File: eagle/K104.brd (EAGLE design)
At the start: 428.3 x 123.6 mm, 229 parts, among them IC1 MAX7219CNG, IC2 MAX7219CNG

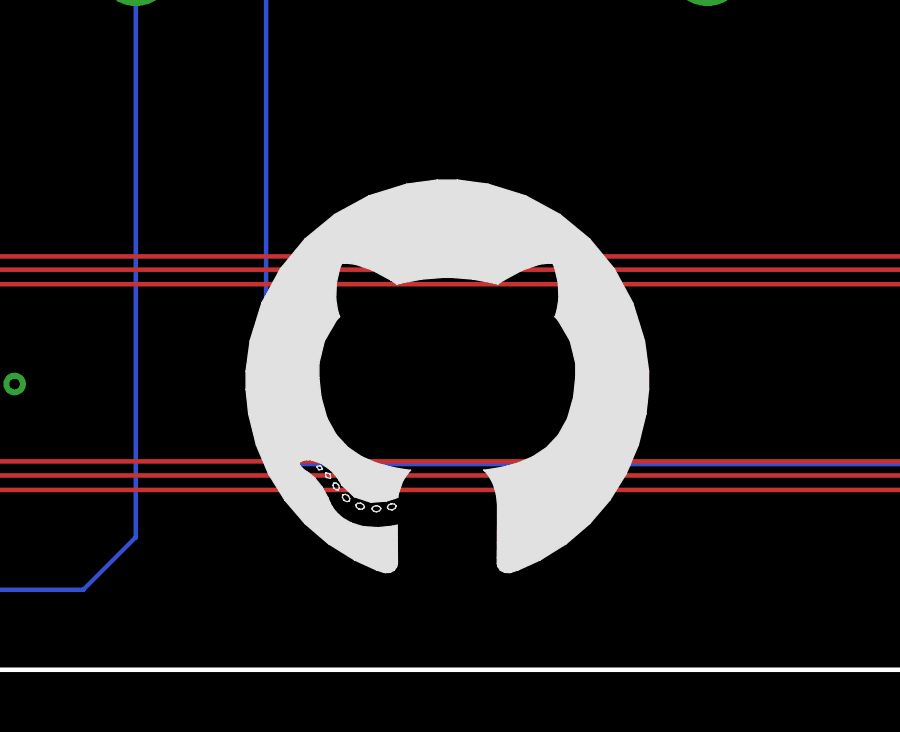
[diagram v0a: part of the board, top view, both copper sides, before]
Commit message: add PCB and case files
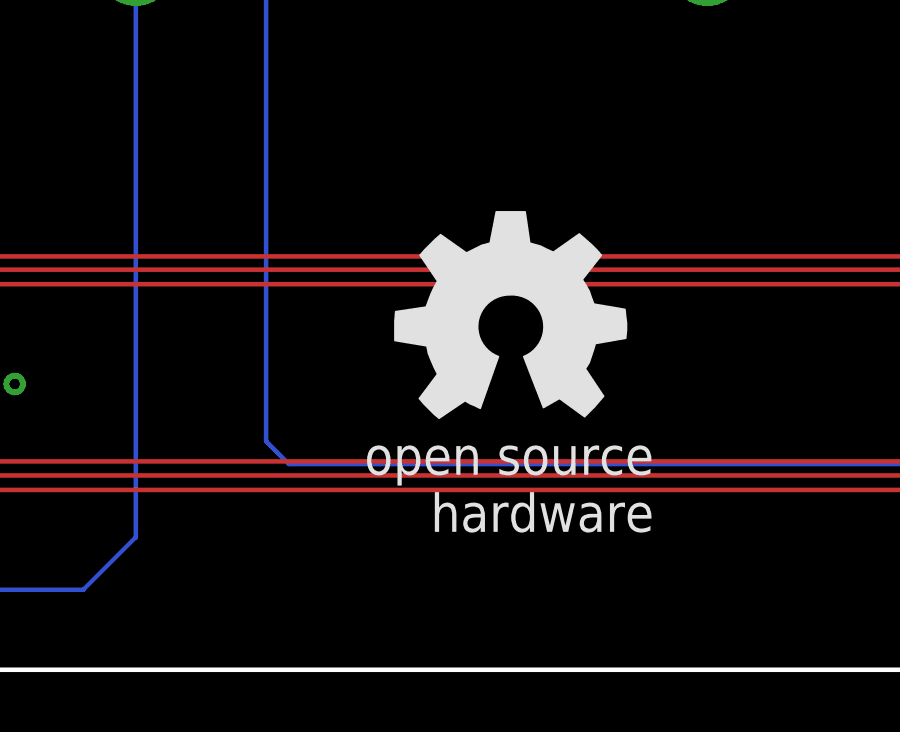
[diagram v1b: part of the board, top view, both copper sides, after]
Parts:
- added U$2, U$3: (no value), oshw:OSHW_8MM
